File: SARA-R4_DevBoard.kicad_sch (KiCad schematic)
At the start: 55 parts, among them J1 JAE_SIM_Card_SF72S006, J2 Battery connector, J3 USB4110-GF-A, J4 SWD connector, SW1 SW_SPDT, U1 SARA-R422X, U2 STM32L432KCUx, U3 ESD224DQAR, U4 MCP73831, U5 SiP32431DR3, U6 TPS7A0218PDBVR, U7 SIM-ST-MFF2, Y1 32.768kHz

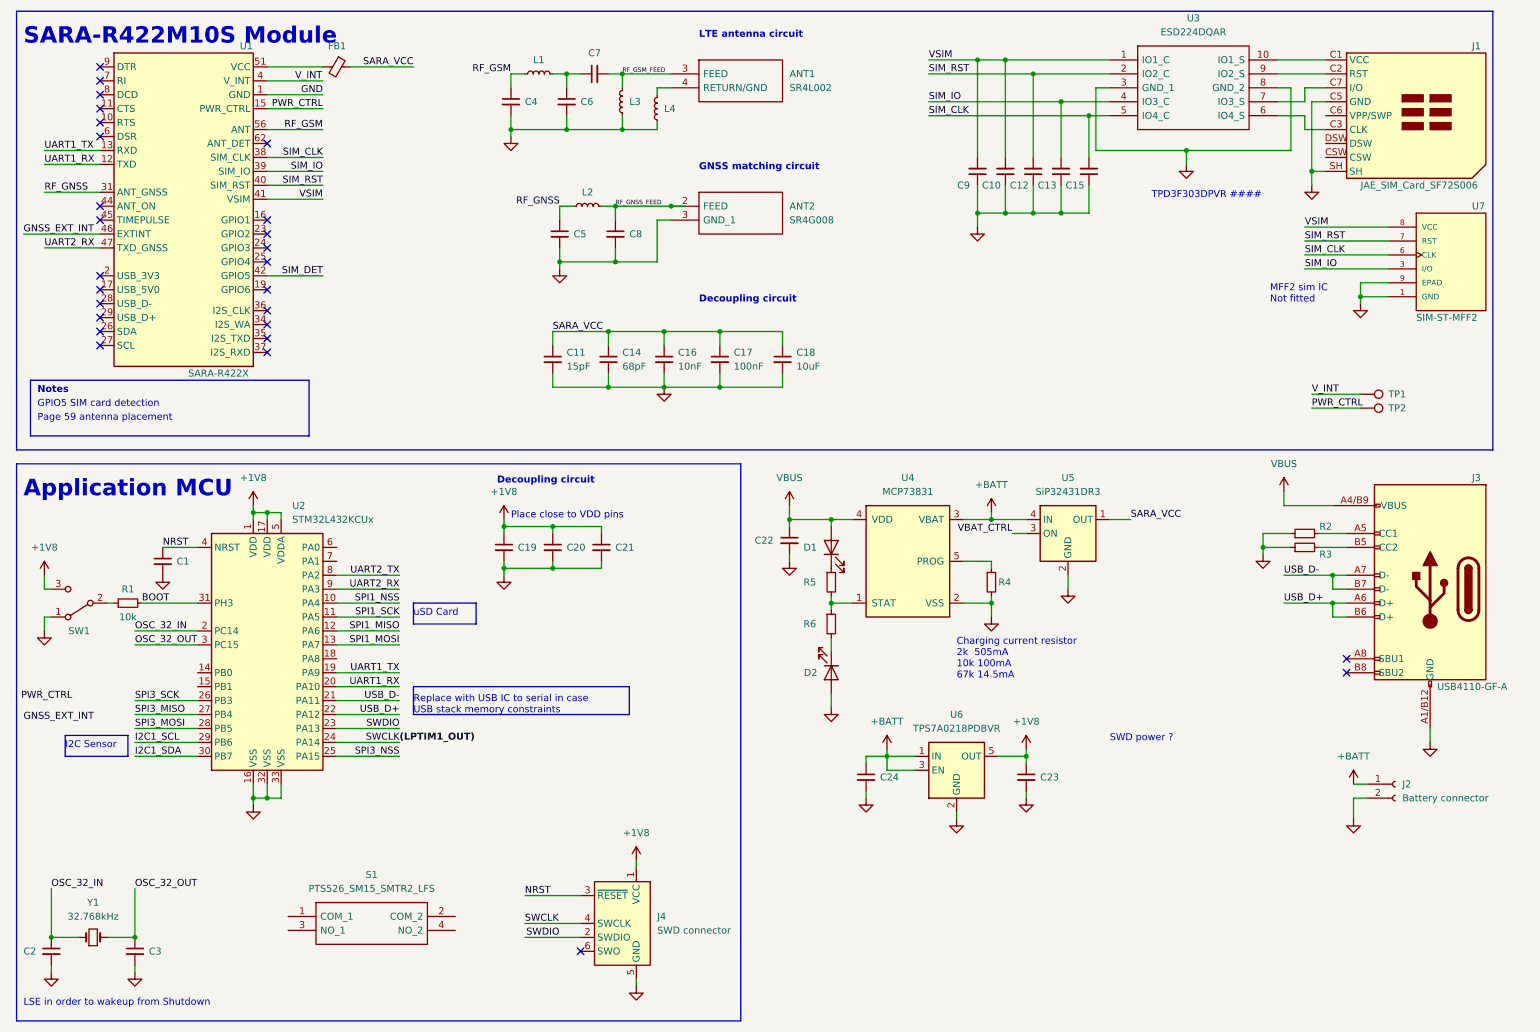
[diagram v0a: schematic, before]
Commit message: Force update
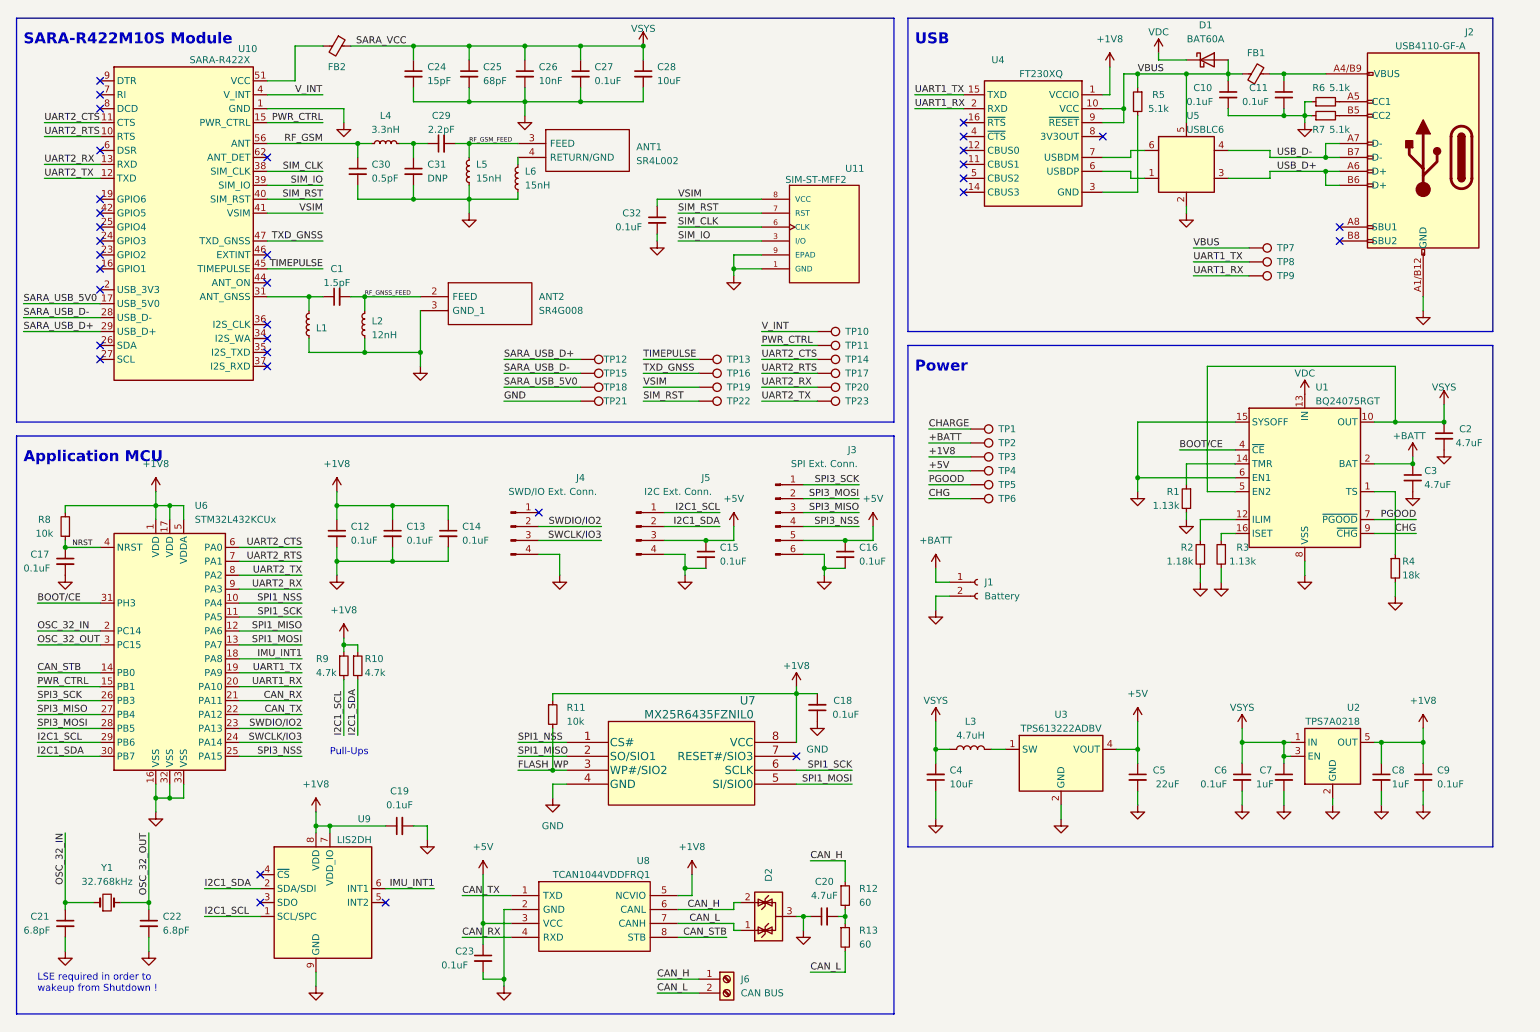
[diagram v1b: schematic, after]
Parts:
- removed C12, C13: 47nF, Capacitor_SMD:C_0402_1005Metric, symbol Device:C_Small
- removed C22: 4.7uF, symbol Device:C_Small
- removed C8: C_Small, Capacitor_SMD:C_0402_1005Metric, symbol Device:C_Small
- removed D1: RED LED, LED_SMD:LED_0402_1005Metric, symbol Device:LED
- removed D2: GREEN LED, LED_SMD:LED_0402_1005Metric, symbol Device:LED
- removed J1: JAE_SIM_Card_SF72S006, Connector_JAE:JAE_SIM_Card_SF72S006, symbol Connector:JAE_SIM_Card_SF72S006
- removed J4: SWD connector, Connector:Tag-Connect_TC2030-IDC-NL_2x03_P1.27mm_Vertical, symbol Connector:Conn_ARM_SWD_TagConnect_TC2030-NL
- removed R6: 470, Resistor_SMD:R_0402_1005Metric, symbol Device:R_Small
- removed S1: PTS526_SM15_SMTR2_LFS, PTS526SM15SMTR2LFS, symbol SARA-R4_DevBoard-lib:PTS526_SM15_SMTR2_LFS
- removed SW1: SW_SPDT, symbol Switch:SW_SPDT
- removed U3: ESD224DQAR, ESD224DQAR, symbol SARA-R4_DevBoard-lib:ESD224DQAR
- removed U4: MCP73831, Package_TO_SOT_SMD:SOT-23-5, symbol Battery_Management:MCP73831-2-OT
- removed U5: SiP32431DR3, Package_TO_SOT_SMD:SOT-363_SC-70-6, symbol Power_Management:SiP32431DR3
- added C1: 1.5pF, Capacitor_SMD:C_0402_1005Metric, symbol Device:C_Small
- added C11, C16, C18, C19, C23, C32, C6: 0.1uF, Capacitor_SMD:C_0402_1005Metric, symbol Device:C_Small
- added C2, C20, C3: 4.7uF, Capacitor_SMD:C_0402_1005Metric, symbol Device:C_Small
- added C4: 10uF, Capacitor_SMD:C_0402_1005Metric, symbol Device:C_Small
- added D1: BAT60A, Diode_SMD:D_SOD-323, symbol Diode:BAT60A
- added D2: SZNUP2115LT1G, Package_TO_SOT_SMD:SOT-23, symbol Power_Protection:NUP2105L
- added FB1: USB_Bead, Inductor_SMD:L_0603_1608Metric, symbol Device:FerriteBead_Small
- added J3: SPI Ext. Conn., Connector_JST:JST_SH_SM06B-SRSS-TB_1x06-1MP_P1.00mm_Horizontal, symbol Connector:Conn_01x06_Male
- added J4: SWD/IO Ext. Conn., Connector_JST:JST_SH_SM04B-SRSS-TB_1x04-1MP_P1.00mm_Horizontal, symbol Connector:Conn_01x04_Male
- added J5: I2C Ext. Conn., Connector_JST:JST_SH_SM04B-SRSS-TB_1x04-1MP_P1.00mm_Horizontal, symbol Connector:Conn_01x04_Male
- added J6: CAN BUS, Capacitor_SMD:C_0603_1608Metric, symbol Connector:Screw_Terminal_01x02
- added L1: L_Small, Inductor_SMD:L_0402_1005Metric, symbol Device:L_Small
- added L3: 4.7uH, Inductor_SMD:L_0402_1005Metric, symbol Device:L
- added R10, R9: 4.7k, Resistor_SMD:R_0402_1005Metric, symbol Device:R_Small
- added R11, R8: 10k, Resistor_SMD:R_0402_1005Metric, symbol Device:R_Small
- added R12, R13: 60, Resistor_SMD:R_0402_1005Metric, symbol Device:R_Small
- added R2: 1.18k, Resistor_SMD:R_0402_1005Metric, symbol Device:R_Small
- added R3: 1.13k, Resistor_SMD:R_0402_1005Metric, symbol Device:R_Small
- added TP1: CHARGE, TestPoint:TestPoint_Pad_D1.0mm, symbol Connector:TestPoint
- added TP12: USB_D+, TestPoint:TestPoint_Pad_D1.0mm, symbol Connector:TestPoint
- added TP13, TP14, TP16, TP17, TP19, TP20, TP22, TP23: TestPoint, TestPoint:TestPoint_Pad_D1.0mm, symbol Connector:TestPoint
- added TP15: USB_D-, TestPoint:TestPoint_Pad_D1.0mm, symbol Connector:TestPoint
- added TP18, TP21: SARA_USB_5V0, TestPoint:TestPoint_Pad_D1.0mm, symbol Connector:TestPoint
- added TP2: BATT, TestPoint:TestPoint_Pad_D1.0mm, symbol Connector:TestPoint
- added TP3: 1V8, TestPoint:TestPoint_Pad_D1.0mm, symbol Connector:TestPoint
- added TP4, TP5, TP6: 5V, TestPoint:TestPoint_Pad_D1.0mm, symbol Connector:TestPoint
- added TP7: VBUS, TestPoint:TestPoint_Pad_D1.0mm, symbol Connector:TestPoint
- added TP8: UART1_TX, TestPoint:TestPoint_Pad_D1.0mm, symbol Connector:TestPoint
- added TP9: UART1_RX, TestPoint:TestPoint_Pad_D1.0mm, symbol Connector:TestPoint
- added U1: BQ24075RGT, Package_DFN_QFN:VQFN-16-1EP_3x3mm_P0.5mm_EP1.6x1.6mm, symbol Battery_Management:BQ24075RGT
- added U3: TPS613222ADBV, Package_TO_SOT_SMD:SOT-23-5, symbol Regulator_Switching:TPS613222ADBV
- added U4: FT230XQ, Package_DFN_QFN:QFN-16-1EP_4x4mm_P0.65mm_EP2.1x2.1mm, symbol Interface_USB:FT230XQ
- added U5: USBLC6, Package_TO_SOT_SMD:SOT-23-6, symbol Power_Protection:USBLC6-2SC6
- added U7: MX25R6435FZNIL0, Package_SON:WSON-8-1EP_4x4mm_P0.8mm_EP2.2x3mm, symbol user_library:MX25R6435FZNIL0
- added U8: TCAN1044VDDFRQ1, SARA-R4_DevBoard_Library:SOT65P280X110-8N, symbol SARA-R4_DevBoard:TCAN1044VDDFRQ1
- added U9: LIS2DH, Package_LGA:LGA-14_2x2mm_P0.35mm_LayoutBorder3x4y, symbol Sensor_Motion:LIS2DH
- ANT1: footprint SARA-R4_DevBoard-lib:SR4L002 -> SARA-R4_DevBoard_Library:SR4L002
- ANT2: footprint SARA-R4_DevBoard-lib:SR4G008 -> SARA-R4_DevBoard_Library:SR4G008
- C10, C15: value 47nF -> 0.1uF; Part GRM1555C1H470JA01 -> (none)
- C12: renamed from C19; value 100nF -> 0.1uF; footprint Capacitor_SMD:C_0603_1608Metric -> Capacitor_SMD:C_0402_1005Metric
- C13: renamed from C20; value 100nF -> 0.1uF; footprint Capacitor_SMD:C_0603_1608Metric -> Capacitor_SMD:C_0402_1005Metric
- C14: renamed from C21; value 100nF -> 0.1uF; footprint Capacitor_SMD:C_0603_1608Metric -> Capacitor_SMD:C_0402_1005Metric
- C17: renamed from C1; value 100nF -> 0.1uF; footprint Capacitor_SMD:C_0603_1608Metric -> Capacitor_SMD:C_0402_1005Metric
- C21: renamed from C2; footprint Capacitor_SMD:C_0603_1608Metric -> Capacitor_SMD:C_0402_1005Metric
- C22: renamed from C3; footprint Capacitor_SMD:C_0603_1608Metric -> Capacitor_SMD:C_0402_1005Metric
- C27: renamed from C17; value 100nF -> 0.1uF; footprint Capacitor_SMD:C_0603_1608Metric -> Capacitor_SMD:C_0402_1005Metric
- C29: renamed from C7; value C_Small -> 2.2pF
- C30: renamed from C4; value C_Small -> 0.5pF; now left out of the parts list
- C31: renamed from C6; now left out of the parts list
- C5: value C_Small -> 22uF
- C7: renamed from C24; footprint Capacitor_SMD:C_0603_1608Metric -> Capacitor_SMD:C_0402_1005Metric
- C8: renamed from C23; footprint Capacitor_SMD:C_0603_1608Metric -> Capacitor_SMD:C_0402_1005Metric
- C9: value 100nF -> 0.1uF; footprint Capacitor_SMD:C_0603_1608Metric -> Capacitor_SMD:C_0402_1005Metric; Part GRM155R71C104KA01 -> (none)
- J1: renamed from J2; value Battery connector -> Battery; footprint Connector_JST:JST_SH_BM02B-SRSS-TB_1x02-1MP_P1.00mm_Vertical -> Connector_JST:JST_PH_S2B-PH-SM4-TB_1x02-1MP_P2.00mm_Horizontal
- J2: renamed from J3; footprint SARA-R4_DevBoard-lib:GCT_USB4110-GF-A_REVB -> SARA-R4_DevBoard_Library:GCT_USB4110-GF-A_REVB
- L2: value L_Small -> 12nH
- R1: value 10k -> 1.13k
- R4: value 2k -> 18k
- R5: value 470 -> 5.1k
- TP10: renamed from TP1; footprint (none) -> TestPoint:TestPoint_Pad_D1.0mm
- TP11: renamed from TP2; footprint (none) -> TestPoint:TestPoint_Pad_D1.0mm
- U11: renamed from U7; footprint SARA-R4_DevBoard-lib:PSON127P500X600X82-9N -> Package_DFN_QFN:DFN-8-1EP_6x5mm_P1.27mm_EP4x4mm; now in the parts list
- U2: renamed from U6; value TPS7A0218PDBVR -> TPS7A0218
- Y1: footprint SARA-R4_DevBoard-lib:NX3215SA32768KEXS00AMU00003 -> SARA-R4_DevBoard_Library:NX3215SA32768KEXS00AMU00003
- renumbered C11 to C24, C14 to C25, C16 to C26, C18 to C28, FB1 to FB2, L1 to L4, L3 to L5, L4 to L6, R2 to R6, R3 to R7, U1 to U10, U2 to U6
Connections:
- net +1V8: now also C9.1, C18.2, C19.1, R10.1, R11.1, R8.2, R9.1, TP3.1, U4.1 (VCCIO), U7.8 (VCC), U8.5 (NCVIO), U9.7 (VDD_IO), U9.8 (VDD)
- net +BATT: now also C3.1, TP2.1, U1.2 (BAT), U1.3 (BAT); no longer C7.1, U2.1 (IN), U2.3 (EN)
- net GND: now also C10.2, C15.2, C9.2, L2.1, R1.2, R5.2, C11.2, C16.2, C18.1, C19.2, C2.2, C20.1, C23.2, C3.2, C32.2, C4.1, C6.2, D2.3 (A), J3.6 (Pin_6), J4.4 (Pin_4), J5.4 (Pin_4), L1.1, R2.2, R3.2, TP21.1, U1.15 (SYSOFF), U1.17 (VSS), U1.6 (EN1), U1.8 (VSS), U3.2 (GND), U4.13 (GND), U4.17 (GND), U4.3 (GND), U5.2 (GND), U7.4 (GND), U8.2 (GND), U9.10 (GND), U9.11 (GND), U9.12 (GND), U9.13 (GND), U9.14 (GND), U9.9 (GND); no longer C10.1, C15.1, C9.1
- net I2C1_SCL: now also J5.1 (Pin_1), R9.2, U9.1 (SCL/SPC)
- net I2C1_SDA: now also J5.2 (Pin_2), R10.2, U9.2 (SDA/SDI)
- net NRST: now also R8.1
- net PWR_CTRL: now also U6.15 (PB1)
- net RF_GNSS_FEED: now also C1.2
- net SIM_CLK: no longer C15.2
- net SIM_RST: now also TP22.1
- net SPI1_MISO: now also U7.2 (SO/SIO1)
- net SPI1_MOSI: now also U7.5 (SI/SIO0)
- net SPI1_NSS: now also U7.1 (CS#)
- net SPI1_SCK: now also U7.6 (SCLK)
- net SPI3_MISO: now also J3.3 (Pin_3)
- net SPI3_MOSI: now also J3.2 (Pin_2)
- net SPI3_NSS: now also J3.4 (Pin_4)
- net SPI3_SCK: now also J3.1 (Pin_1)
- net UART1_RX: now also TP9.1, U4.2 (RXD); no longer U10.12 (TXD)
- net UART1_TX: now also TP8.1, U4.15 (TXD); no longer U10.13 (RXD)
- net UART2_RX: now also U10.13 (RXD), TP20.1; no longer U10.47 (TXD_GNSS)
- net UART2_TX: now also U10.12 (TXD), TP23.1
- net USB_D+: now also U5.3 (I/O2); no longer U6.22 (PA12)
- net USB_D-: now also U5.4 (I/O2); no longer U6.21 (PA11)
- net VBUS: now also C10.1, R5.1, D1.2 (A), FB1.1, TP7.1, U4.10 (VCC), U4.9 (~{RESET}), U5.5 (VBUS); no longer J2.A4/B9 (VBUS), J2.B4/A9 (VBUS)
- net VSIM: now also C32.1, TP19.1; no longer C10.2, C9.2
- net CAN_STB: now reaches U6.14 (PB0)
- net CAN_STB: now also U8.8 (STB)
- net IMU_INT1: now reaches U6.18 (PA8)
- net IMU_INT1: now also U9.6 (INT1)
- net UART2_CTS: now reaches U6.6 (PA0)
- net UART2_CTS: now also U10.11 (CTS), TP14.1
- net UART2_RTS: now reaches U6.7 (PA1)
- net UART2_RTS: now also U10.10 (RTS), TP17.1
- net at R1.1: now also U1.14 (TMR)
- net at R4.1: now also U1.1 (TS)
- net SARA_USB_5V0: now reaches U10.17 (USB_5V0)
- net SARA_USB_5V0: now also TP18.1
- net SARA_USB_D-: now reaches U10.28 (USB_D-)
- net SARA_USB_D-: now also TP15.1
- net SARA_USB_D+: now reaches U10.29 (USB_D+)
- net SARA_USB_D+: now also TP12.1
- net TIMEPULSE: now reaches U10.45 (TIMEPULSE)
- net TIMEPULSE: now also TP13.1
- net (LPTIM1_OUT) renamed SWCLK/IO3
- net SWCLK/IO3: now also J4.3 (Pin_3)
- net BOOT renamed BOOT/CE
- net BOOT/CE: now also U1.4 (~{CE}); no longer R1.2
- net GNSS_EXT_INT: no longer names the net of U10.46 (EXTINT)
- removed net RF_GNSS: C5.1, L2.1, U10.31 (ANT_GNSS)
- net SARA_VCC renamed VSYS
- net VSYS: now also C7.1, U2.1 (IN), U2.3 (EN), C2.1, C4.2, C6.1, L3.2, U1.10 (OUT), U1.11 (OUT), U1.5 (EN2)
- net SIM_DET: no longer names the net of U10.42 (GPIO5)
- net SWDIO renamed SWDIO/IO2
- net SWDIO/IO2: now also J4.2 (Pin_2)
- new net: R2.1, U1.12 (ILIM)
- new net: R3.1, U1.16 (ISET)
- new net: C1.1, L1.2, U10.31 (ANT_GNSS)
- new net: L3.1, U3.1 (SW)
- new net: C20.2, R12.2, R13.1
- new net: C11.1, FB1.2, J2.A4/B9 (VBUS), J2.B4/A9 (VBUS)
- new net: U4.6 (USBDP), U5.1 (I/O1)
- new net: U4.7 (USBDM), U5.6 (I/O1)
- new net +5V: C15.1, C16.1, C23.1, C5.1, J3.5 (Pin_5), J5.3 (Pin_3), TP4.1, U3.4 (VOUT), U8.3 (VCC)
- new net CAN_H: D2.2 (K), J6.1 (Pin_1), R12.1, U8.6 (CANL)
- new net CAN_L: D2.1 (K), J6.2 (Pin_2), R13.2, U8.7 (CANH)
- new net CAN_RX: U6.21 (PA11), U8.4 (RXD)
- new net CAN_TX: U6.22 (PA12), U8.1 (TXD)
- new net CHARGE: TP1.1
- new net CHG: TP6.1, U1.9 (~{CHG})
- new net FLASH_WP: R11.2, U7.3 (WP#/SIO2)
- new net PGOOD: TP5.1, U1.7 (~{PGOOD})
- new net TXD_GNSS: TP16.1, U10.47 (TXD_GNSS)
- new net VDC: D1.1 (K), U1.13 (IN)
- no-connect marks 27 -> 34
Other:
- note added: "LSE required in order to wakeup from Shutdown !"
- note added: "Power"
- note added: "Pull-Ups"
- note added: "USB"
- note removed: "Charging current resistor 2k 505mA 10k 100mA 67k 14.5mA"
- note removed: "Decoupling circuit"
- note removed: "GNSS matching circuit"
- note removed: "GPIO5 SIM card detection"
- note removed: "I2C Sensor"
- note removed: "LSE in order to wakeup from Shutdown"
- note removed: "LTE antenna circuit"
- note removed: "MFF2 sim IC Not fitted"
- note removed: "Notes"
- note removed: "Page 59 antenna placement"
- note removed: "Place close to VDD pins"
- note removed: "Replace with USB IC to serial in case USB stack memory constraints"
- note removed: "SWD power ?"
- note removed: "TPD3F303DPVR ####"
- note removed: "uSD Card"
- title: SARA-R4 Tracker -> SARA-R4 Development board
- moved on the sheet: ANT1, ANT2, C12, C13, C14, C17, C21, C22, C24, C25, C26, C27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
